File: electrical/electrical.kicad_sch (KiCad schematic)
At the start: 0 parts

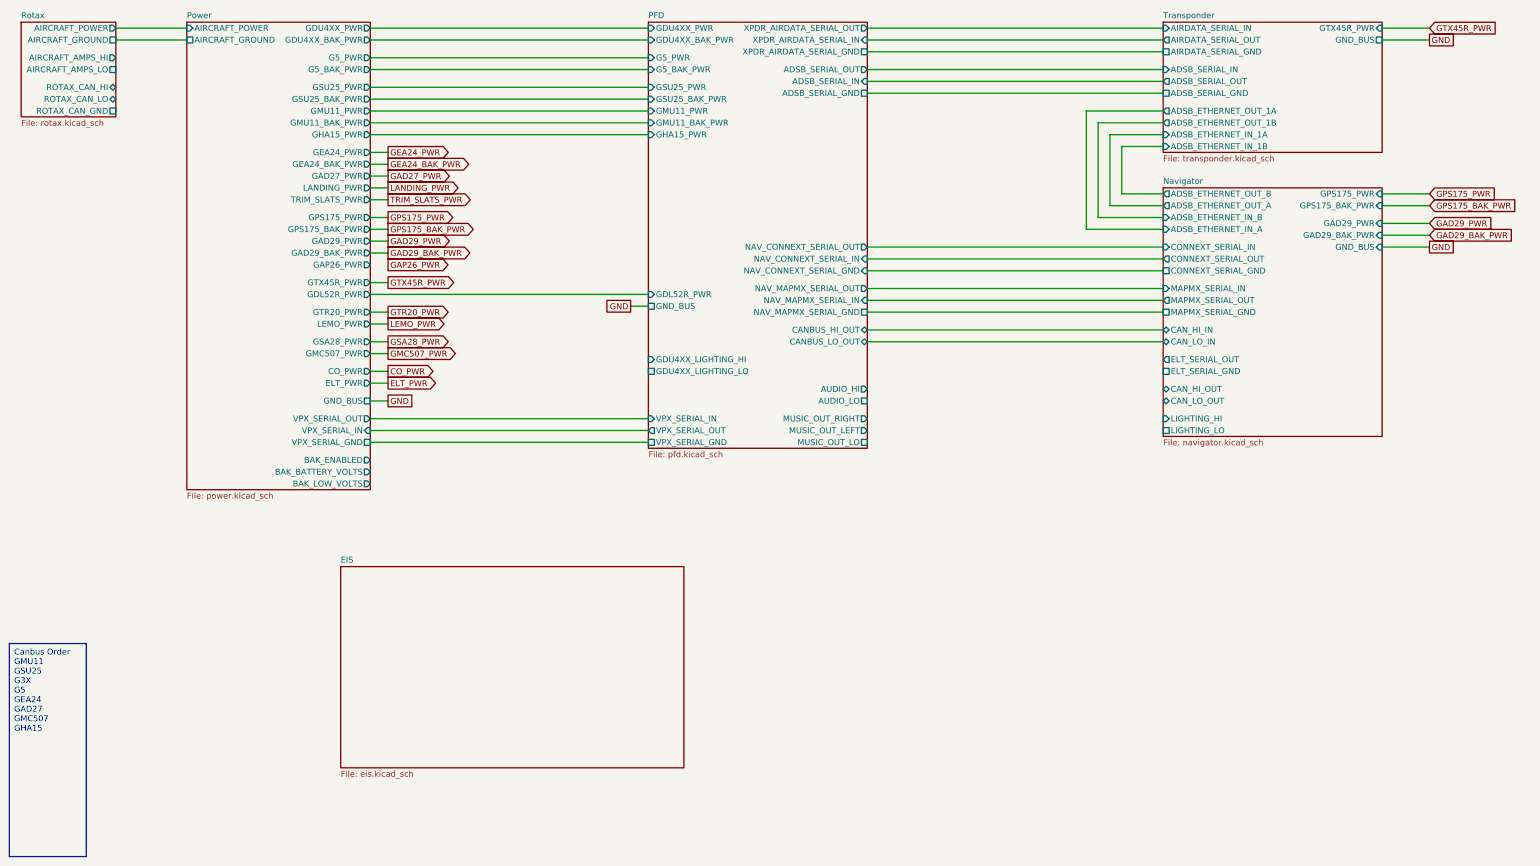
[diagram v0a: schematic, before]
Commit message: Added EIS
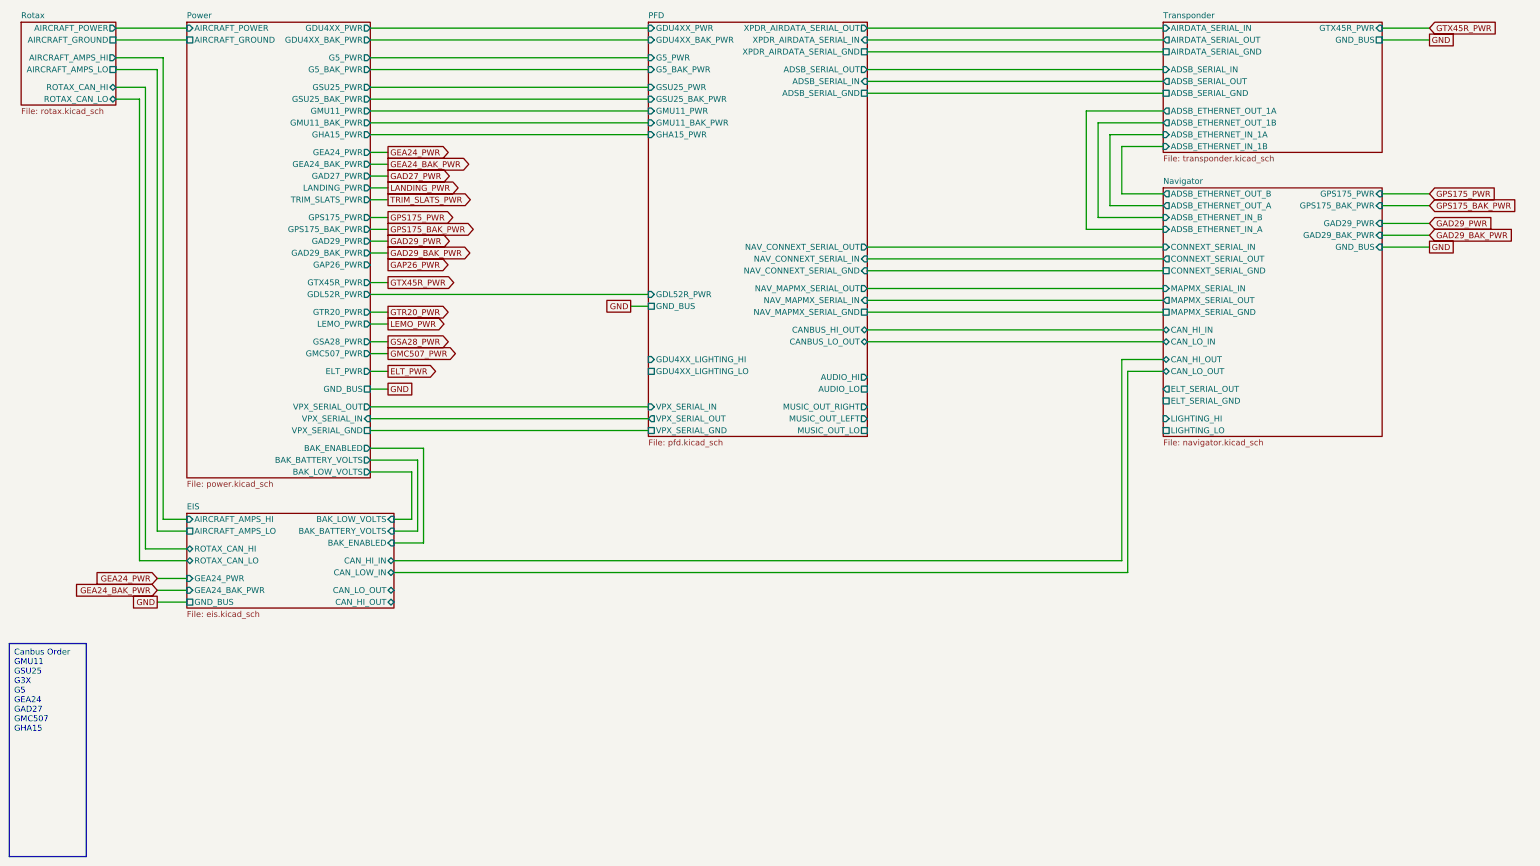
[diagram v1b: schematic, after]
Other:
- sheet EIS ports: added AIRCRAFT_AMPS_HI, AIRCRAFT_AMPS_LO, BAK_BATTERY_VOLTS, BAK_ENABLED, BAK_LOW_VOLTS, CAN_HI_IN, CAN_HI_OUT, CAN_LOW_IN, CAN_LO_OUT, GEA24_BAK_PWR, GEA24_PWR, GND_BUS, ROTAX_CAN_HI, ROTAX_CAN_LO; removed none
- sheet Power ports: added none; removed CO_PWR
- sheet Rotax ports: added none; removed ROTAX_CAN_GND

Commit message: Added Multifunction
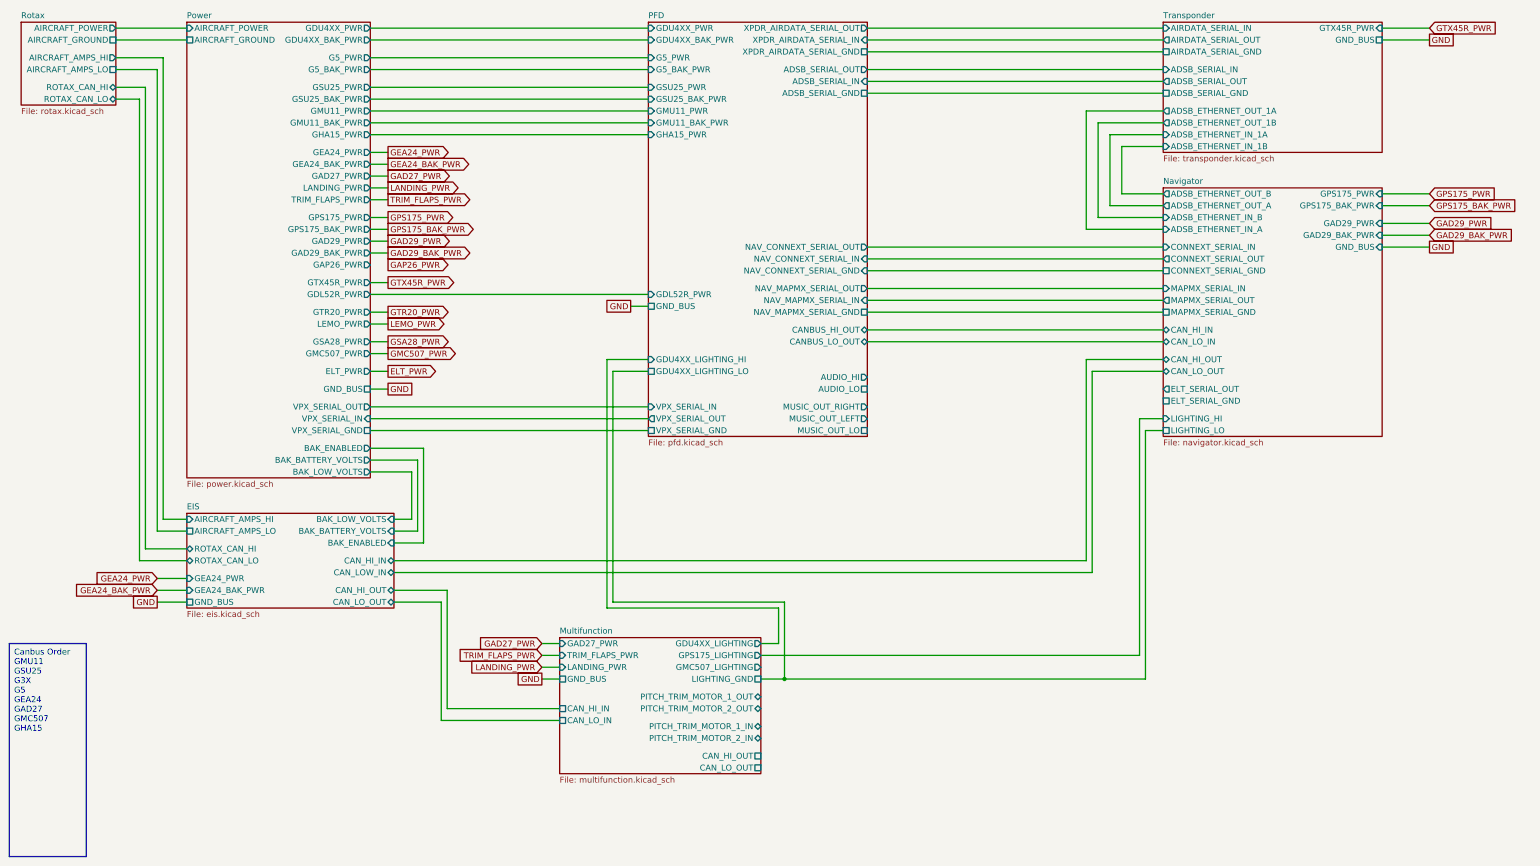
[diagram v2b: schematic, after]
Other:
- added sheet Multifunction (multifunction.kicad_sch)
- sheet Power ports: added TRIM_FLAPS_PWR; removed TRIM_SLATS_PWR
